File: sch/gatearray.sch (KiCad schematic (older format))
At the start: 78 parts, among them X2 CONN-7S

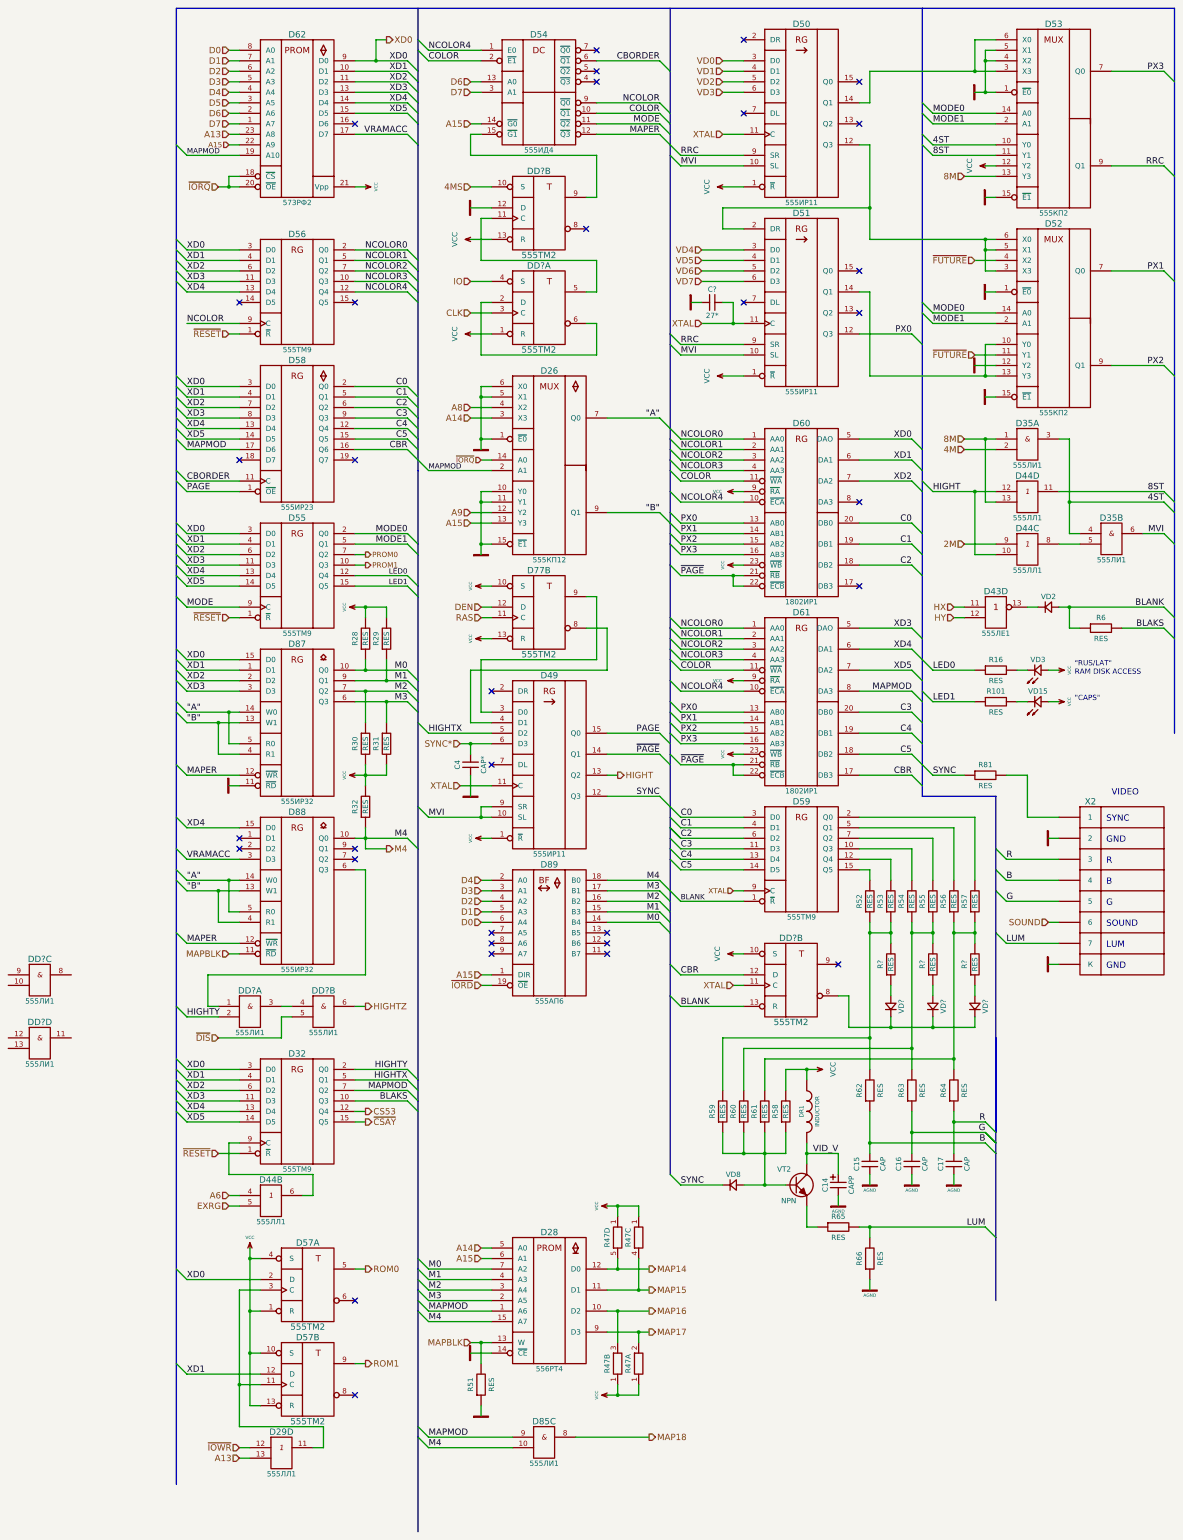
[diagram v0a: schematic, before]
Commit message: GAL based PLL for FDC
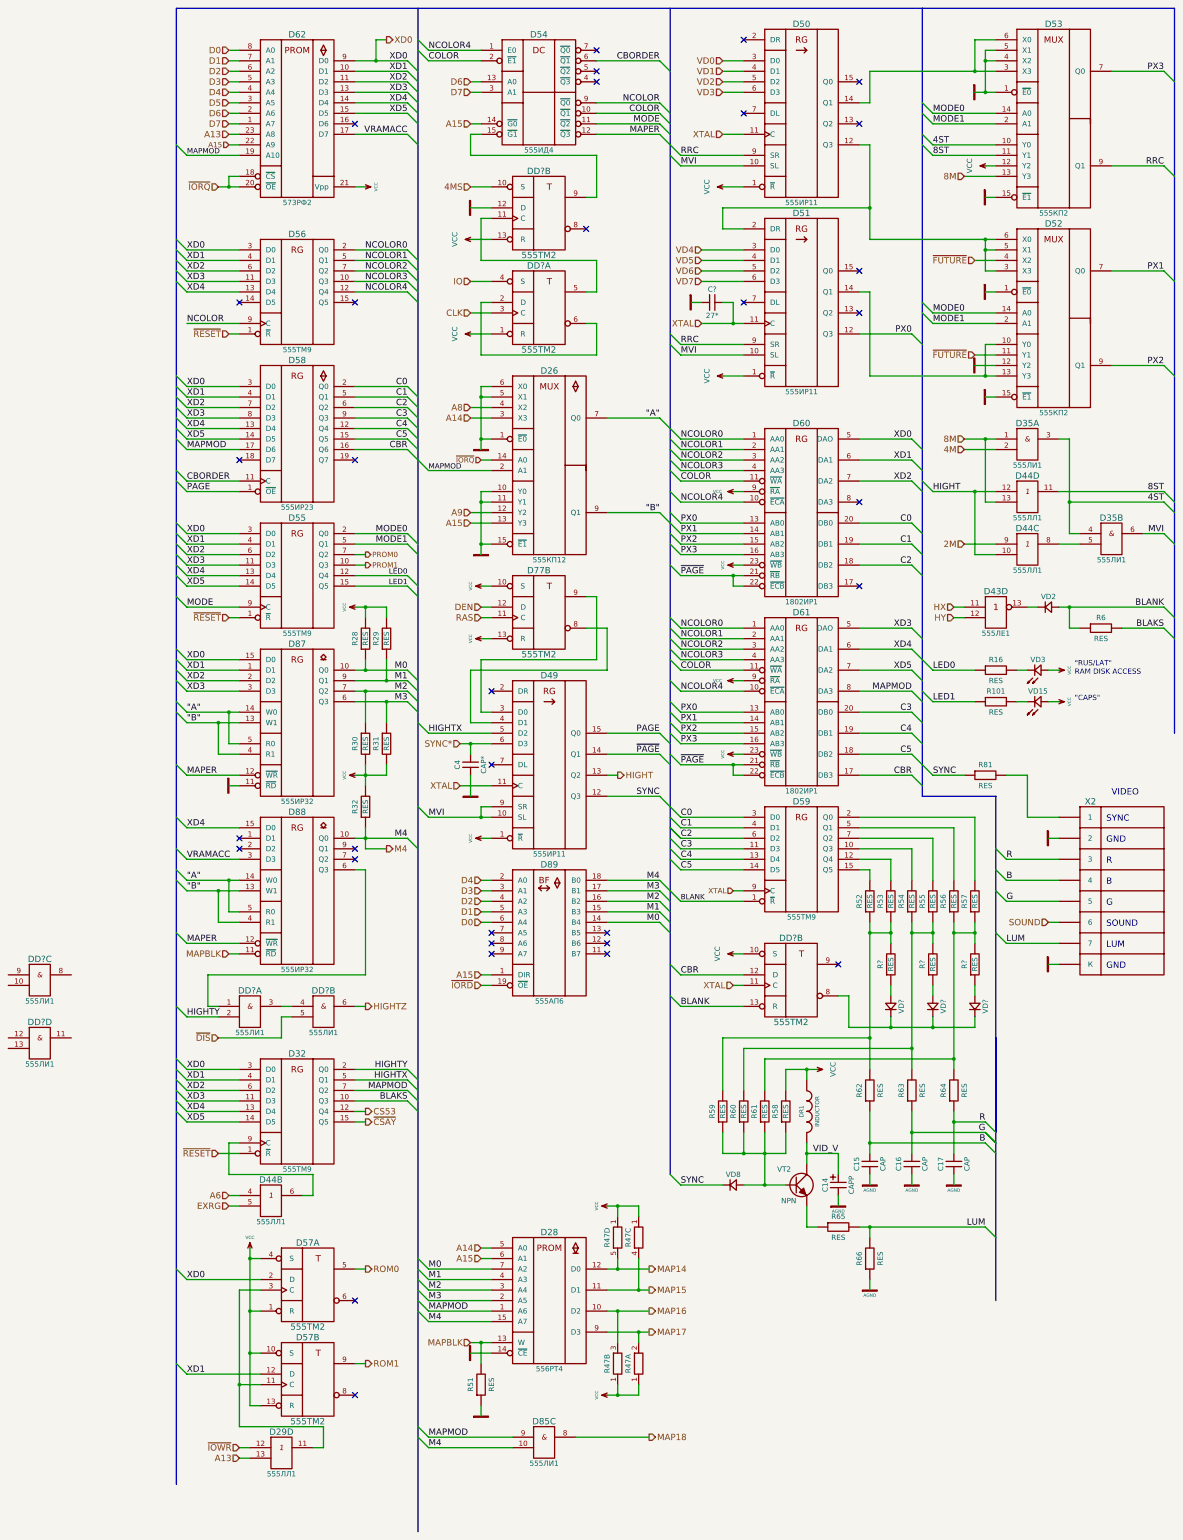
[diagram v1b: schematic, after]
